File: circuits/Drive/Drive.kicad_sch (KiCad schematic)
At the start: 23 parts, among them J1 Conn_01x14_Pin, SW1 SW_SPST, U1 STM32F446VETx, Y1 16MHz

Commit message: Driveほぼ完成
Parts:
- removed C10, C15: 0.1uF, Capacitor_SMD:C_0402_1005Metric, symbol Device:C
- removed C12, C13: 2.2uF, Capacitor_SMD:C_0402_1005Metric, symbol Device:C
- removed C14: 4.7uF, Capacitor_SMD:C_0603_1608Metric, symbol Device:C
- removed R3: 1k, Resistor_SMD:R_0402_1005Metric, symbol Device:R
- removed U1: STM32F446VETx, Package_QFP:LQFP-100_14x14mm_P0.5mm, symbol MCU_ST_STM32F4:STM32F446VETx
- removed Y1: 16MHz, Crystal:Crystal_SMD_3225-4Pin_3.2x2.5mm_HandSoldering, symbol Device:Crystal_GND24
- added R62: 1k, Resistor_SMD:R_0402_1005Metric, symbol Device:R
- added U2: STM32F446RETx, Package_QFP:LQFP-64_10x10mm_P0.5mm, symbol MCU_ST_STM32F4:STM32F446RETx
- added Y2: 16MHz, Crystal:Crystal_SMD_3225-4Pin_3.2x2.5mm, symbol Device:Crystal_GND24
- C11: value 1uF -> 4.7uF; footprint Capacitor_SMD:C_0402_1005Metric -> Capacitor_SMD:C_0603_1608Metric
- C9: value 0.1uF -> 1uF
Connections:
- net +3.3V: now also C9.2, U2.1 (VBAT), U2.13 (VDDA), U2.19 (VDD), U2.32 (VDD), U2.48 (VDD), U2.64 (VDD); no longer C11.1, C9.1
- net BOOT0: now also U2.60 (BOOT0)
- net GNDD: now also C9.1, R62.2, U2.12 (VSSA), U2.18 (VSS), U2.31 (VSS), U2.47 (VSS), U2.63 (VSS), Y2.2, Y2.4; no longer C9.2
- net HSE_IN: now also U2.5 (PH0), Y2.1
- net HSE_OUT: now also U2.6 (PH1), Y2.3
- net NRST: now also U2.7 (NRST)
- net SWCLK: now also U2.49 (PA14)
- net SWDIO: now also U2.46 (PA13)
- net SWO: now also U2.55 (PB3)
- net at R2.1: now also U2.28 (PB2)
- net VBUS: no longer names the net of D1.1 (K), J1.3 (Pin_3)
- net VBUS: now also R62.1
- new net: C11.1, U2.30 (VCAP_1)
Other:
- sheet RS485 renamed RS485_RingNW
- added sheet RS485_MD (RS485_MD.kicad_sch)
- sheet RS485_RingNW: file RS485.kicad_sch -> RS485_RingNW.kicad_sch
- sheet RS485_RingNW ports: added MainRX_RS485RingX_TX, MainRX_RS485RingY_TX, MainTX_RS485RingX_RX, MainTX_RS485RingY_RX; removed MainRX_RS485Bst_TX, MainRX_RS485Cam_TX, MainRX_RS485MD_TX, MainRX_RS485Spr_TX, MainRX_RS485UI_TX, MainTX_RS485Bst_RX, MainTX_RS485Cam_RX, MainTX_RS485MD_RX, MainTX_RS485Spr_RX, MainTX_RS485UI_RX
- sheet UI ports: added DIP_SW0, DIP_SW1, DIP_SW2, DIP_SW3; removed Slide_SW1, Tact_SW0
- note added: "F446RE"
- note removed: "F446VE"
- moved on the sheet: C1, C2, C3, C4, C5, C6, C7, R1, R2, SW1

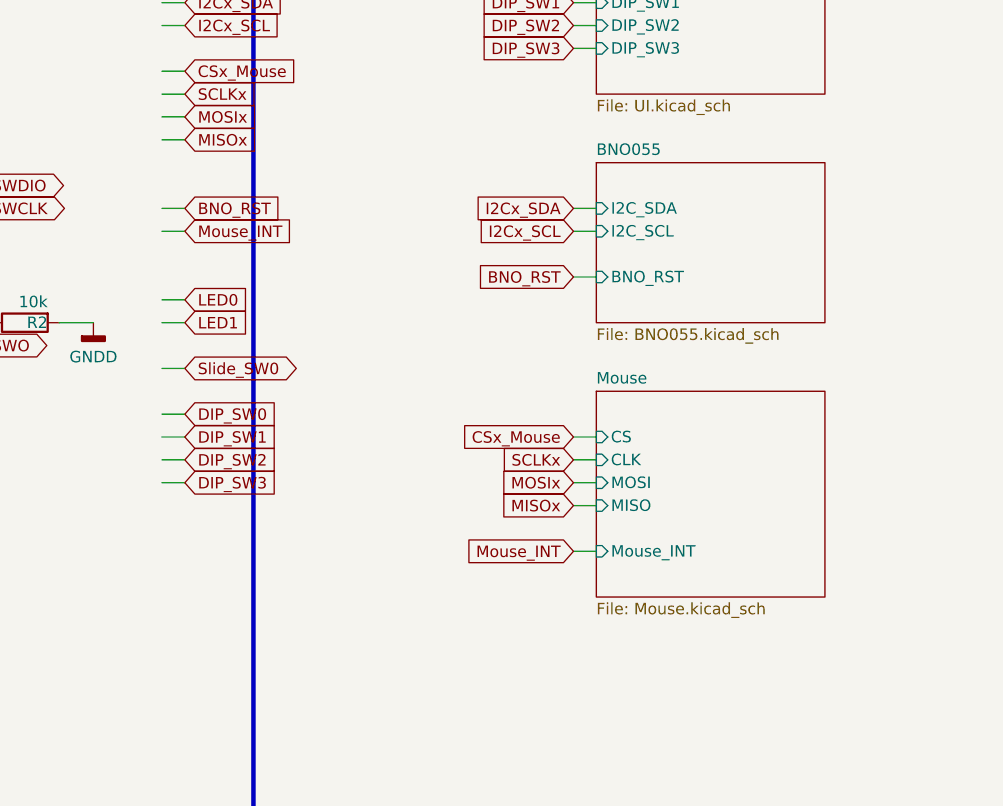
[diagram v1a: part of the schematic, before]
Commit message: 無線&UI完成？
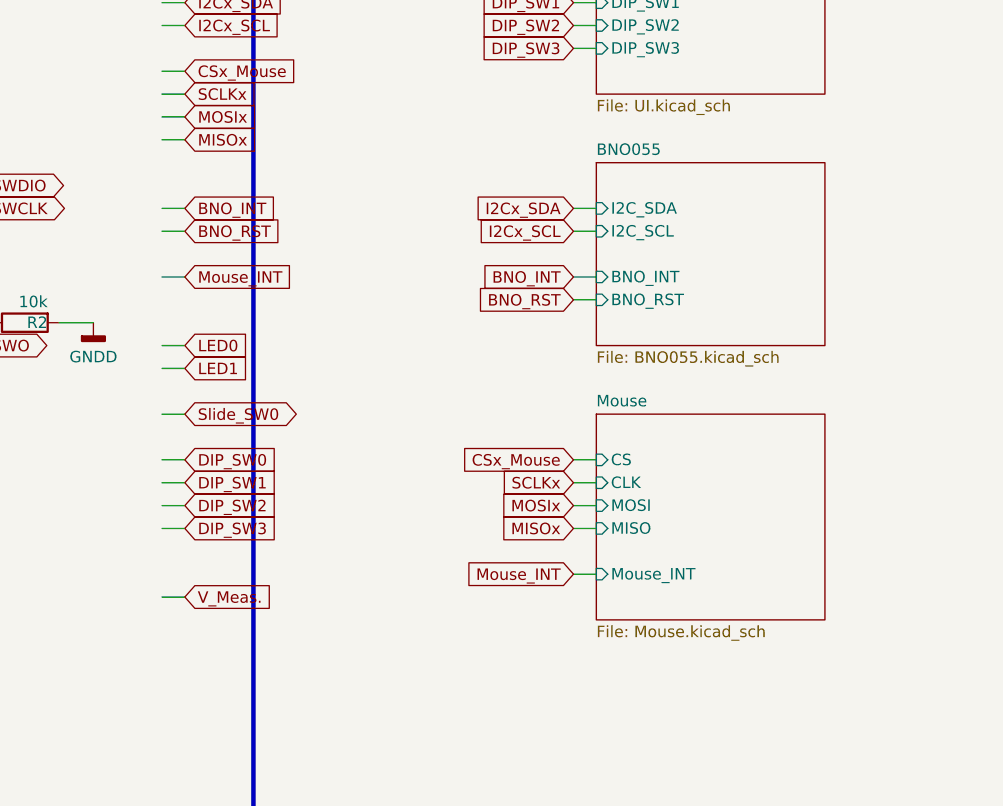
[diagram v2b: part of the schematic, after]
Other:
- sheet BNO055 ports: added BNO_INT; removed none

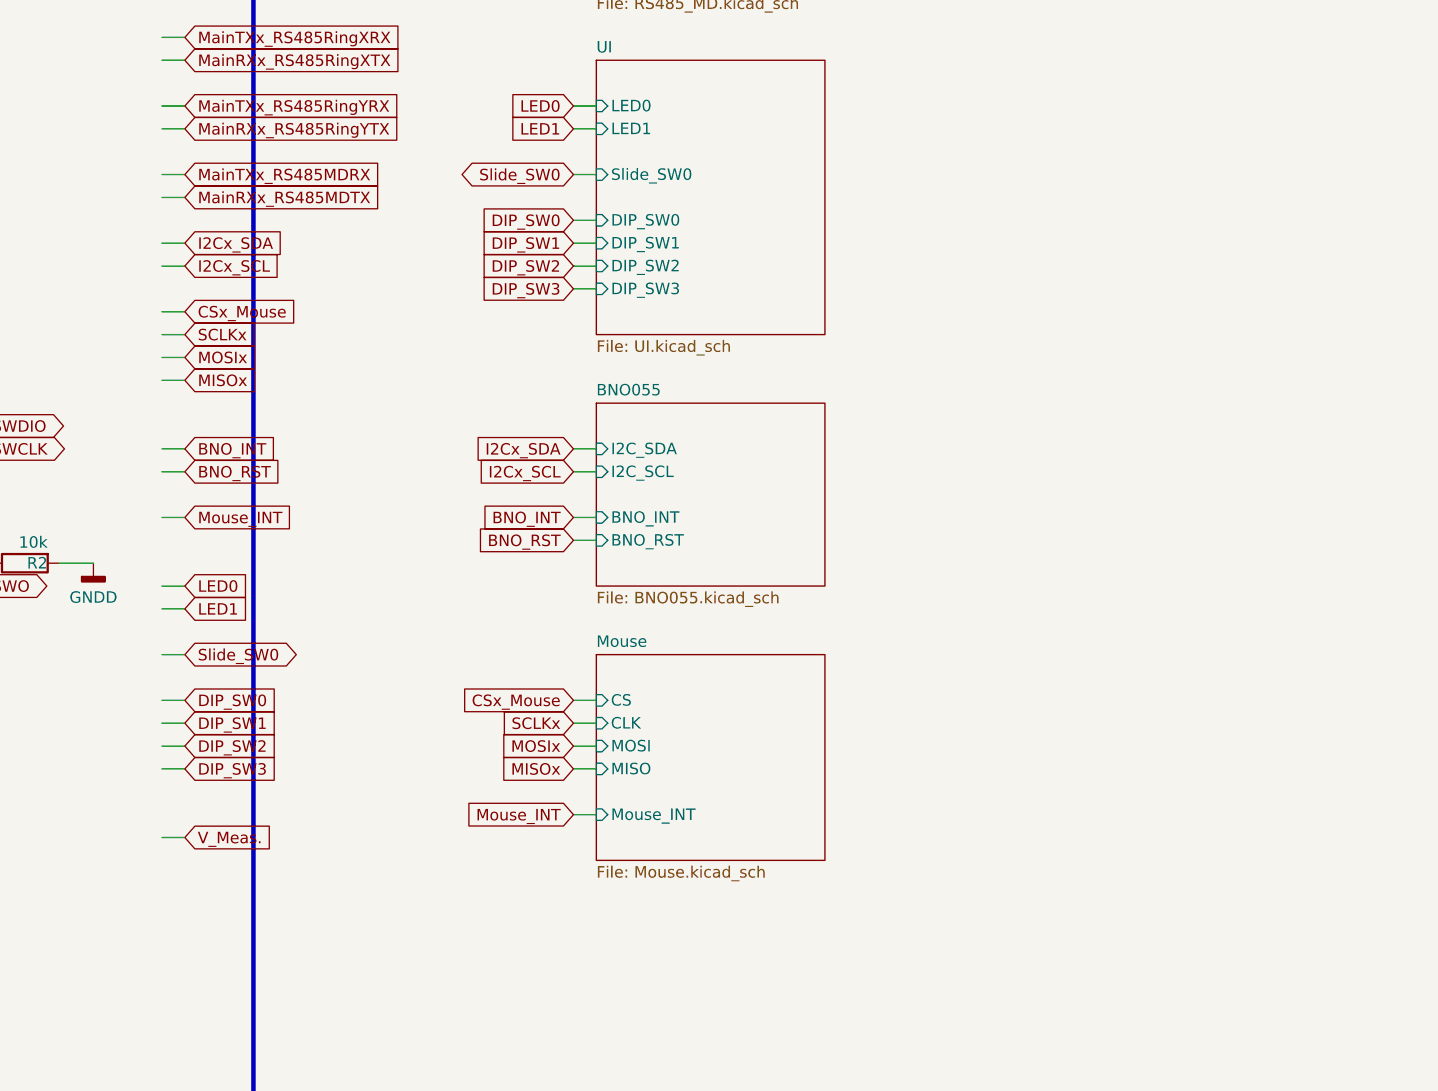
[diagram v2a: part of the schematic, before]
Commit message: ラズパイ基板とか
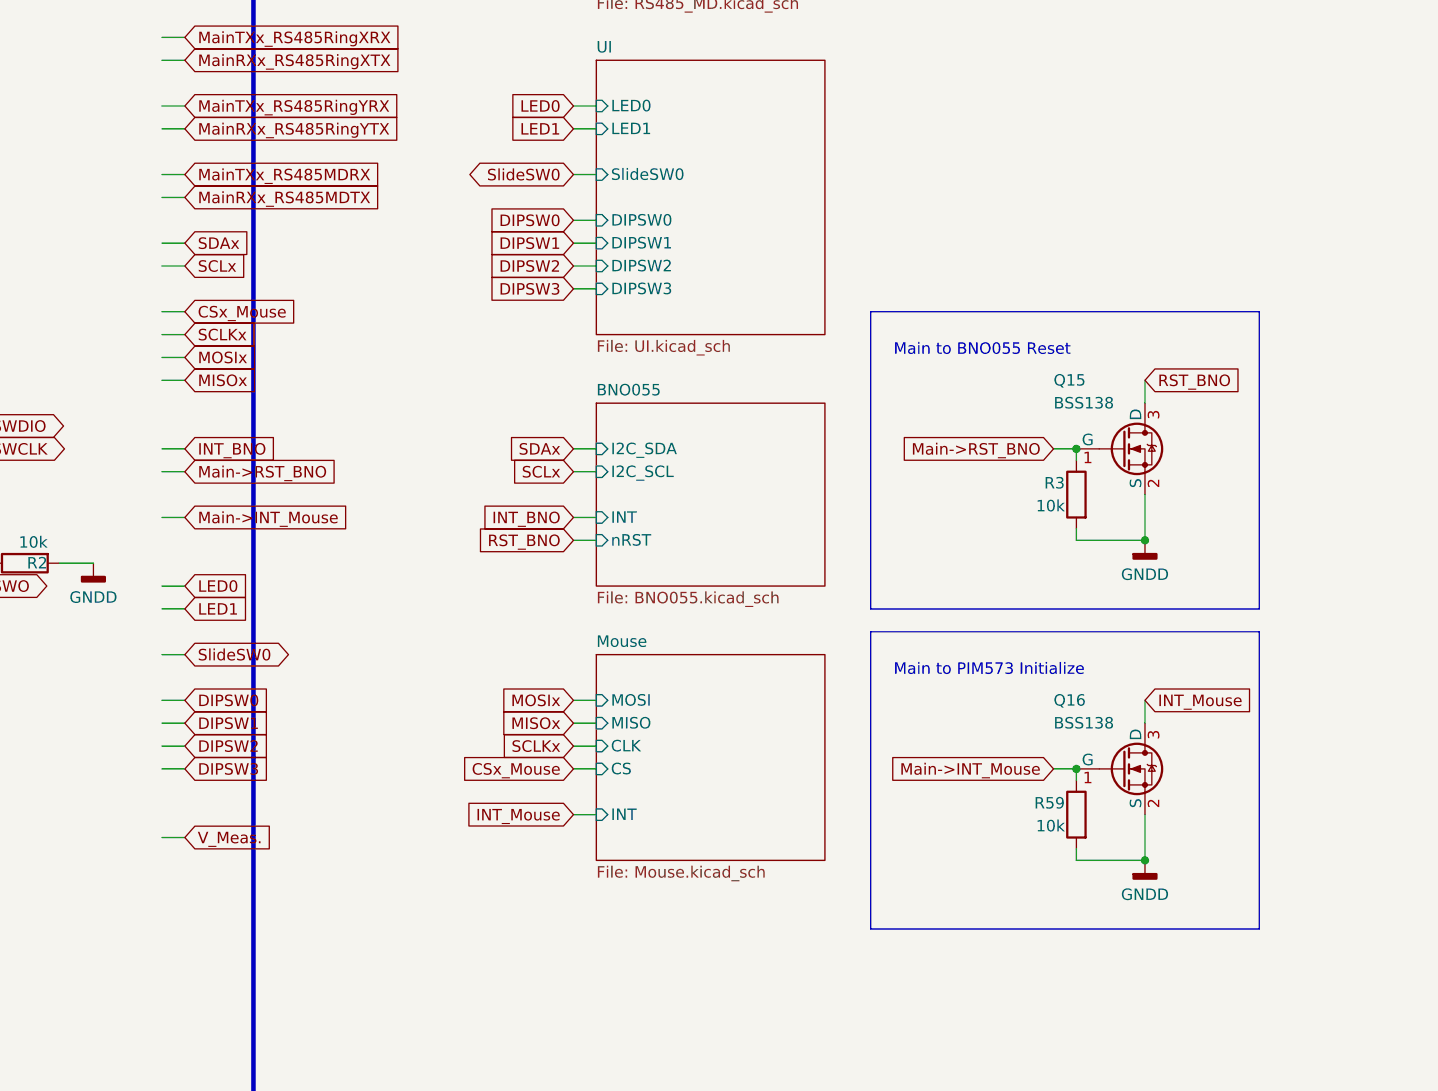
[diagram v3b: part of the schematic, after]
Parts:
- added Q15, Q16: BSS138, Package_TO_SOT_SMD:SOT-23, symbol Device:Q_NMOS_GSD
- added R3, R59: 10k, Resistor_SMD:R_0402_1005Metric, symbol Device:R
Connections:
- net GNDD: now also Q15.2 (S), Q16.2 (S), R3.2, R59.2
- new net INT_Mouse: Q16.3 (D)
- new net Main->INT_Mouse: Q16.1 (G), R59.1
- new net Main->RST_BNO: Q15.1 (G), R3.1
- new net RST_BNO: Q15.3 (D)
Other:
- sheet BNO055 ports: added INT, nRST; removed BNO_INT, BNO_RST
- sheet Mouse ports: added INT; removed Mouse_INT
- sheet UI ports: added DIPSW0, DIPSW1, DIPSW2, DIPSW3, SlideSW0; removed DIP_SW0, DIP_SW1, DIP_SW2, DIP_SW3, Slide_SW0
- note added: "Main to BNO055 Reset"
- note added: "Main to PIM573 Initialize"

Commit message: PDFプロット
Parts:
- added C10: 0.1uF, Capacitor_SMD:C_0402_1005Metric, symbol Device:C
- added R68: 10k, Resistor_SMD:R_0402_1005Metric, symbol Device:R
- added SW5: SW_SPST, symbol Switch:SW_SPST
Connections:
- net +3.3V: now also C10.1, SW5.2 (B)
- net GNDD: now also R68.2
- new net SHDN/BOOT: C10.2, R68.1, SW5.1 (A)
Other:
- sheet UI ports: added LED_B0, LED_B1, LED_LG0, LED_Y0, LED_nR0; removed LED0, LED1
- note added: "ShutDown/BOOT Switch"
- moved on the sheet: C1, C11, C2, C3, C4, C5, C6, C7, C9, D1, J1, Q15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
